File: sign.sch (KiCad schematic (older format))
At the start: 169 parts, among them J1 CONN_01X02, J10 CONN_01X02, J11 CONN_01X02, J12 CONN_01X02, J13 CONN_01X02, J14 CONN_01X02, J15 CONN_01X02, J16 CONN_01X02, J17 CONN_01X02, J18 CONN_01X02, J19 CONN_01X02, J2 CONN_01X02, J20 CONN_01X02, J21 CONN_01X02, J22 CONN_01X02, J23 CONN_01X02, J24 CONN_01X02, J25 CONN_01X02, J26 CONN_01X02, J27 CONN_01X02, J28 CONN_01X02, J29 CONN_01X02, J3 CONN_01X02, J30 CONN_01X02, J4 CONN_01X02, J5 CONN_01X02, J6 CONN_01X02, J7 CONN_01X02, J8 CONN_01X02, J9 CONN_01X02, U1 APA102C_x6, U10 APA102C_x2, U100 APA102C_x6, U101 APA102C_x4, U102 APA102C_x2, U103 APA102C_x1, U104 APA102C_x3, U105 APA102C_x5, U106 APA102C_x2, U107 APA102C_x3, U108 APA102C_x10, U109 APA102C_x9, U11 APA102C_x2, U110 APA102C_x3, U111 APA102C_x12, U112 APA102C_x16, U113 APA102C_x8, U114 APA102C_x13, U115 APA102C_x3, U116 APA102C_x6, U117 APA102C_x3, U118 APA102C_x6, U119 APA102C_x3, U12 APA102C_x2, U120 APA102C_x2, U121 APA102C_x6, U122 APA102C_x3, U123 APA102C_x6, U124 APA102C_x7, U125 APA102C_x12, U126 APA102C_x6, U127 APA102C_x11, U128 APA102C_x4, U129 APA102C_x6, U13 APA102C_x2, U130 APA102C_x2, U131 APA102C_x2, U132 APA102C_x3, U133 APA102C_x1, U134 APA102C_x3, U135 APA102C_x3, U136 APA102C_x12, U137 APA102C_x12, U138 APA102C_x9, U139 APA102C_x4, U14 APA102C_x3, U15 APA102C_x3, U16 APA102C_x3, U17 APA102C_x3, U18 APA102C_x5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

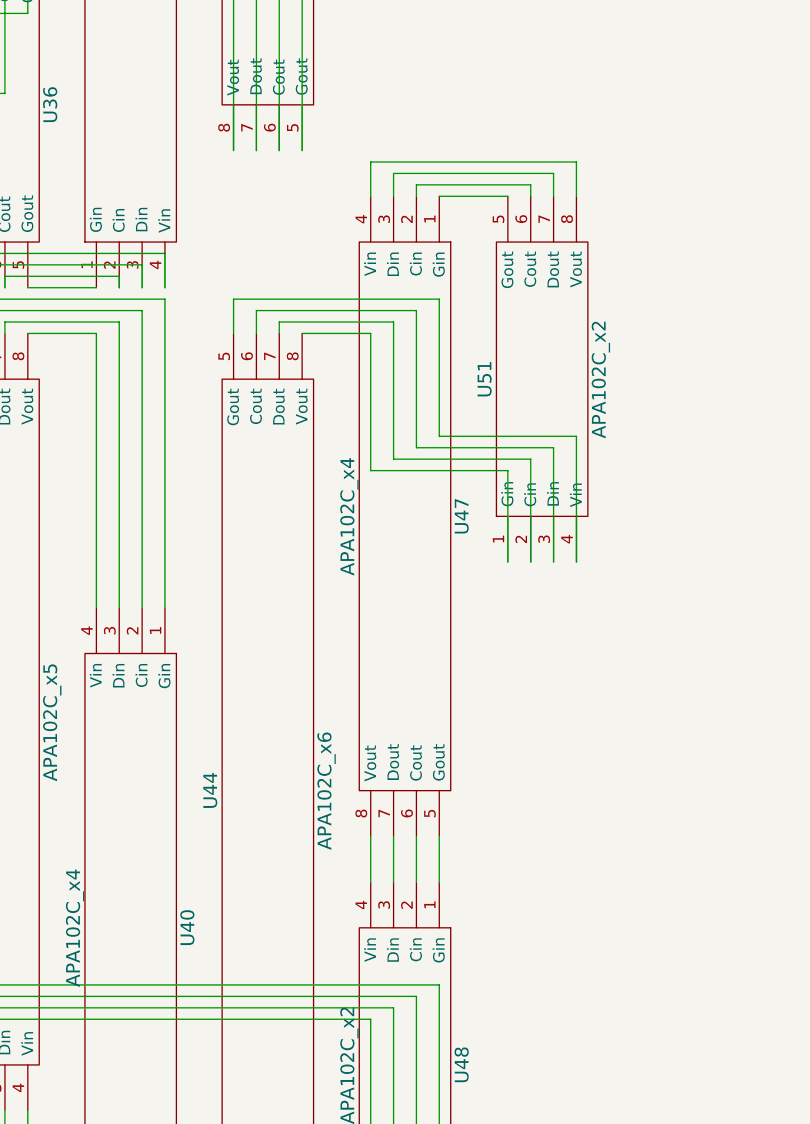
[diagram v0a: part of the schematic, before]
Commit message: finish all the tracks
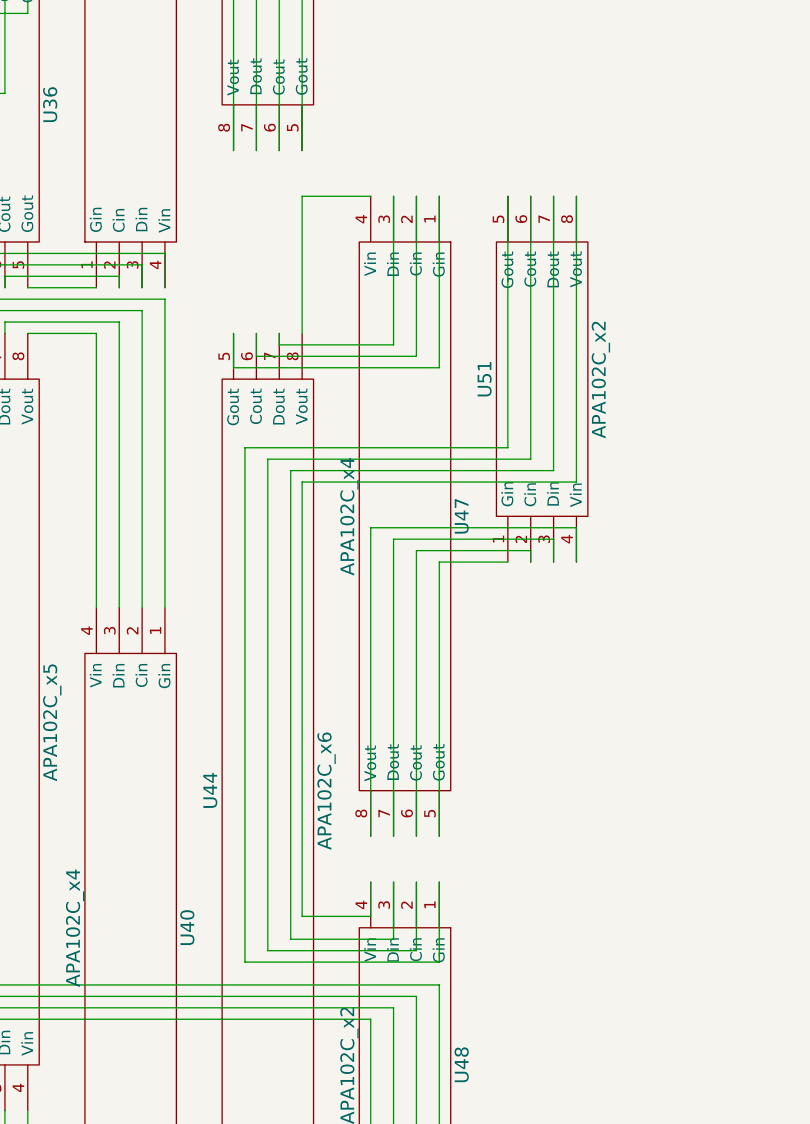
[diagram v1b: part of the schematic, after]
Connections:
- net at U44.5 (Gout): now also U47.1 (Gin); no longer U51.4 (Vin)
- net at U44.6 (Cout): now also U47.2 (Cin); no longer U51.3 (Din)
- net at U44.7 (Dout): now also U47.3 (Din); no longer U51.2 (Cin)
- net at U44.8 (Vout): now also U47.4 (Vin); no longer U51.1 (Gin)
- net at U51.5 (Gout): now also U48.1 (Gin); no longer U47.1 (Gin)
- net at U51.6 (Cout): now also U48.2 (Cin); no longer U47.2 (Cin)
- net at U51.7 (Dout): now also U48.3 (Din); no longer U47.3 (Din)
- net at U51.8 (Vout): now also U48.4 (Vin); no longer U47.4 (Vin)
- net at U47.5 (Gout): now also U51.1 (Gin); no longer U48.1 (Gin)
- net at U47.6 (Cout): now also U51.2 (Cin); no longer U48.2 (Cin)
- net at U47.7 (Dout): now also U51.3 (Din); no longer U48.3 (Din)
- net at U47.8 (Vout): now also U51.4 (Vin); no longer U48.4 (Vin)
